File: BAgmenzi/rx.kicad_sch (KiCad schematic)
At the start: 37 parts, among them IC1 TPL0501-100RSER, U2 AD8338ACPZ-R7, U3 OPA836IDBVT, U4 OPA836IDBVT, U5 TPS22916CYFPR, U6 TPS22916CYFPR

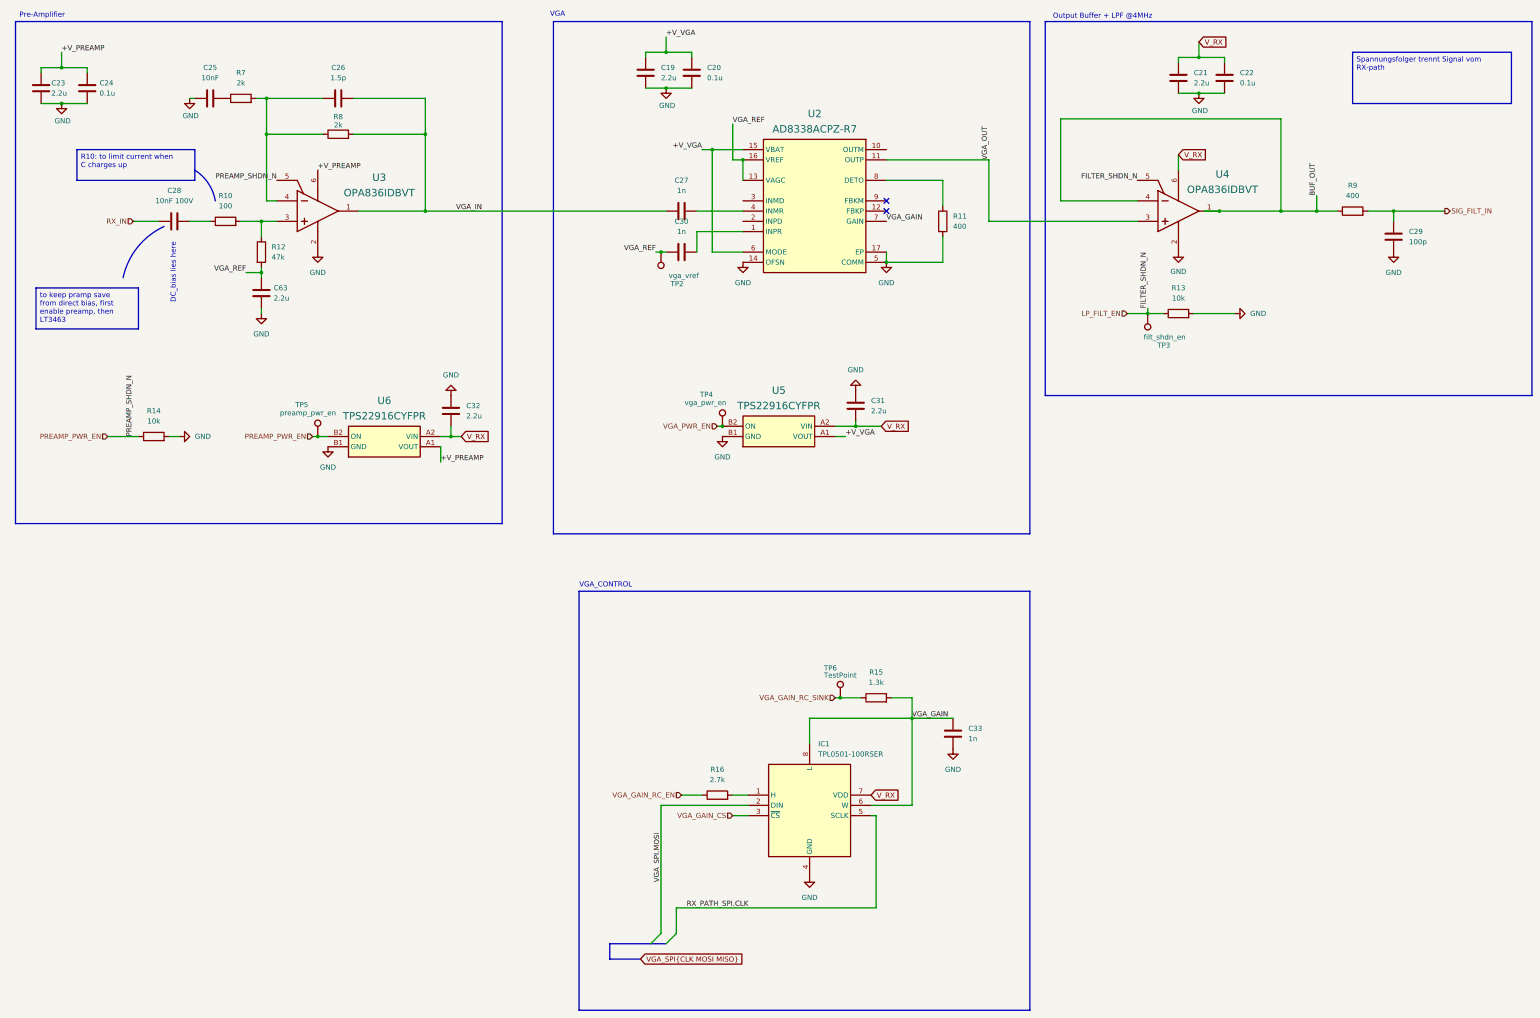
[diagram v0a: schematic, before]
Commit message: added libraries, other changes in sch, started pcb
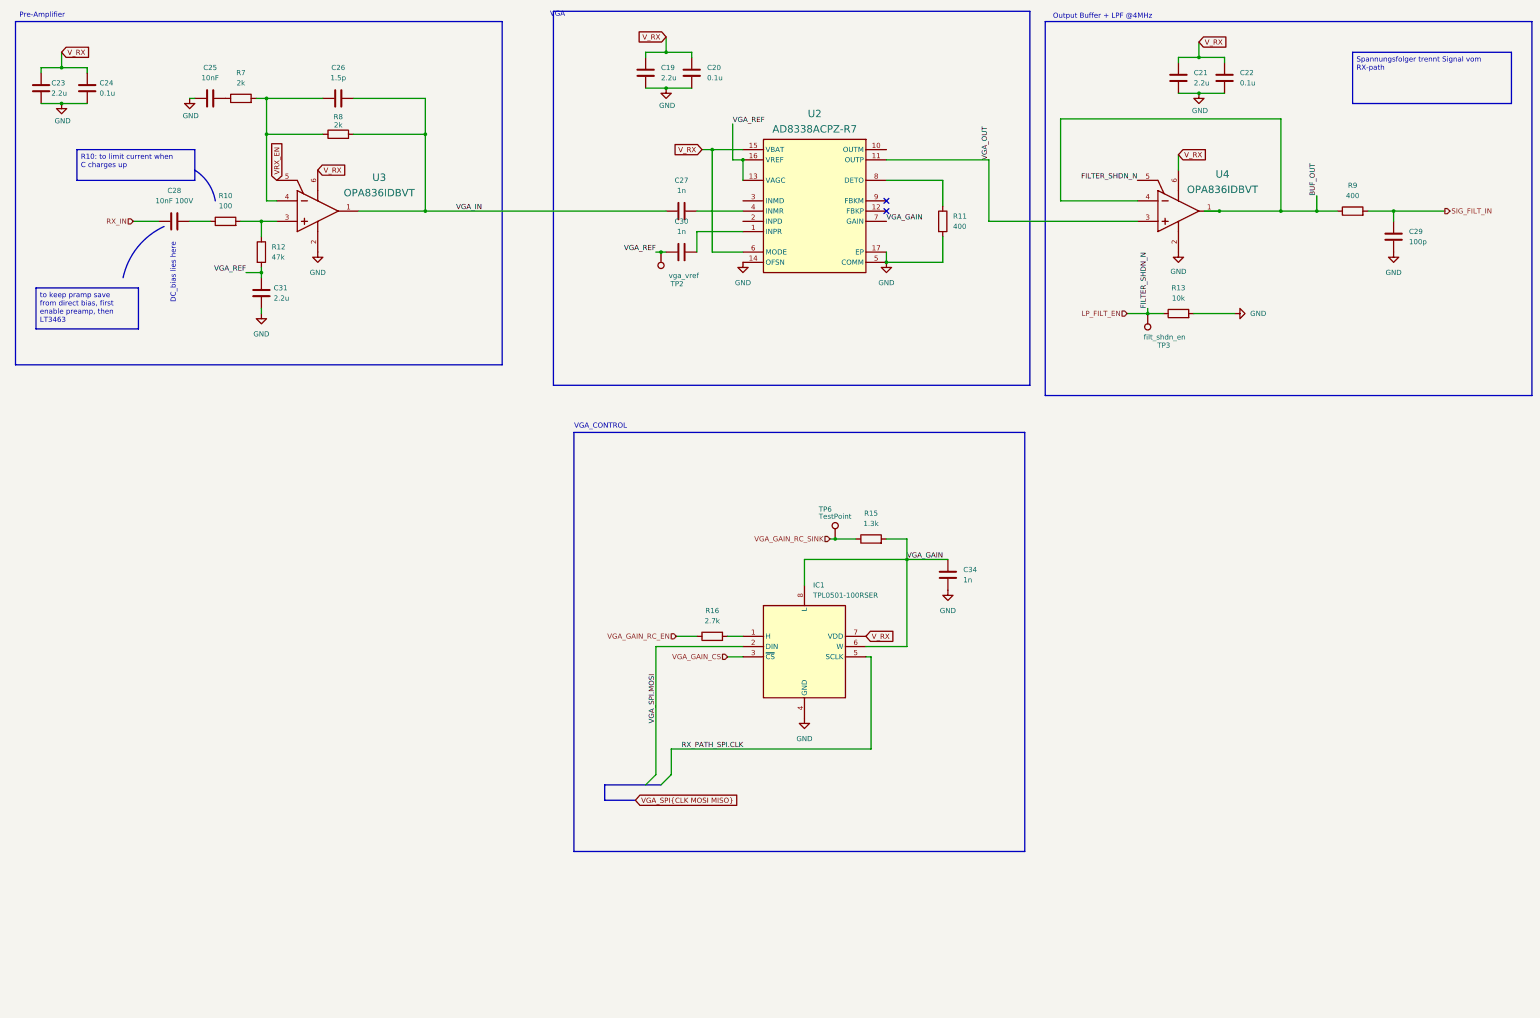
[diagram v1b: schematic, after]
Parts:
- removed C31, C32: 2.2u, symbol Device:C
- removed R14: 10k, symbol Device:R
- removed TP4: vga_pwr_en, symbol Connector:TestPoint
- removed TP5: preamp_pwr_en, symbol Connector:TestPoint
- removed U5: TPS22916CYFPR, BGA4C40P2X2_78X78X50:BGA4C40P2X2_78X78X50, symbol TPS22916CYFPR:TPS22916CYFPR
- removed U6: TPS22916CYFPR, BGA4C40P2X2_78X78X50, symbol TPS22916CYFPR:TPS22916CYFPR
- C19, C20, C21, C22, C23, C24, C25, C26, C27, C29, C30: footprint (none) -> Capacitor_SMD:C_0402_1005Metric
- C28: footprint Capacitor_SMD:C_0201_0603Metric -> Capacitor_SMD:C_0402_1005Metric
- C31: renamed from C63; footprint (none) -> Capacitor_SMD:C_0402_1005Metric
- C34: renamed from C33; footprint (none) -> Capacitor_SMD:C_0402_1005Metric
- IC1: footprint RSE0008A -> KiCad:RSE0008A
- R10, R11, R12, R13, R15, R16, R7, R8, R9: footprint (none) -> Resistor_SMD:R_0402_1005Metric
- TP2: footprint (none) -> TestPoint:TestPoint_Loop_D2.50mm_Drill1.85mm
- TP6: footprint (none) -> TestPoint:TestPoint_Loop_D2.50mm_Drill1.0mm_LowProfile
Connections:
- net +V_PREAMP is gone; now on net V_RX: C23.2, C24.2, U3.6 (VS+)
- net +V_VGA is gone; now on net V_RX: C19.2, C20.2, U2.15 (VBAT), U2.6 (MODE)
- net PREAMP_PWR_EN renamed VRX_EN
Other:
- moved on the sheet: C34, IC1, R15, R16, TP6
